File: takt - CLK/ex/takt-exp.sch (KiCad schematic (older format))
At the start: 55 parts, among them J1 PJ301M-12, J2 PJ301M-12, J3 PJ301M-12, J4 PJ301M-12, J5 PJ301M-12, J6 PJ301M-12, J7 PJ301M-12, J8 PJ301M-12, J9 PJ301M-12, Q1 2N3904, Q2 2N3904, Q3 2N3904, SW1 SW_SP3T, SW2 SW_SP3T, SW3 SW_SP3T, U1 TL074, U2 TL074, U3 TL074, U4 ATmega328P-PU

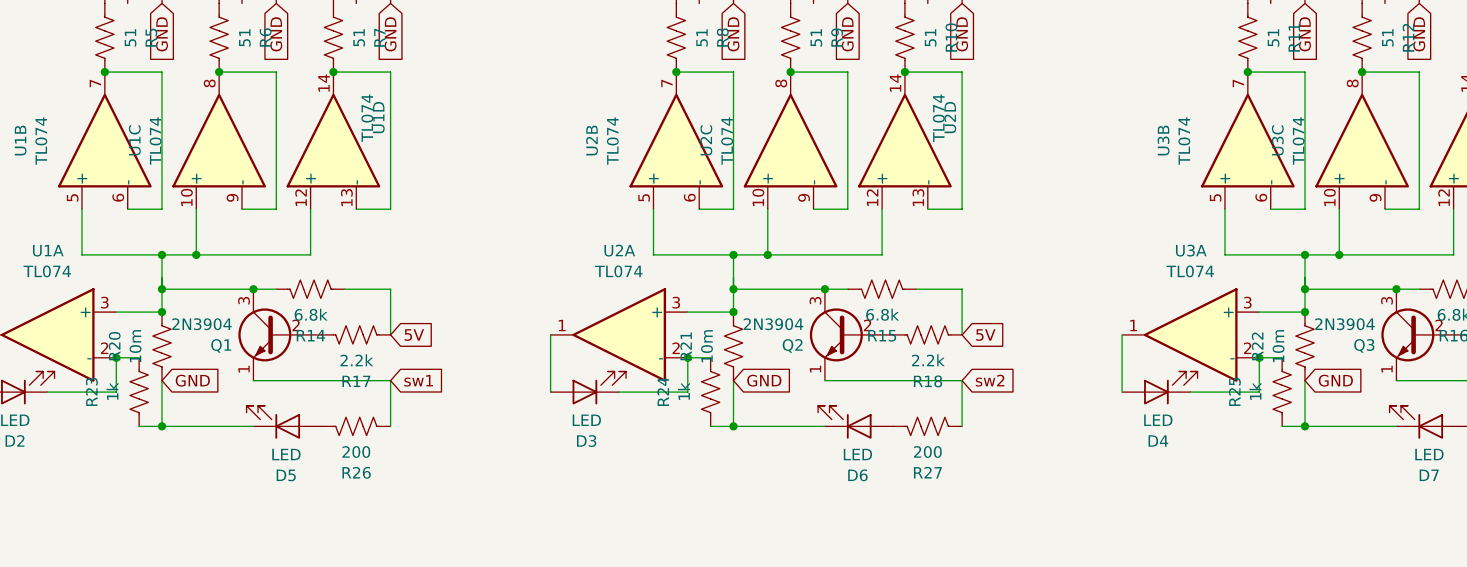
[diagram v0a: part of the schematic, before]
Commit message: update
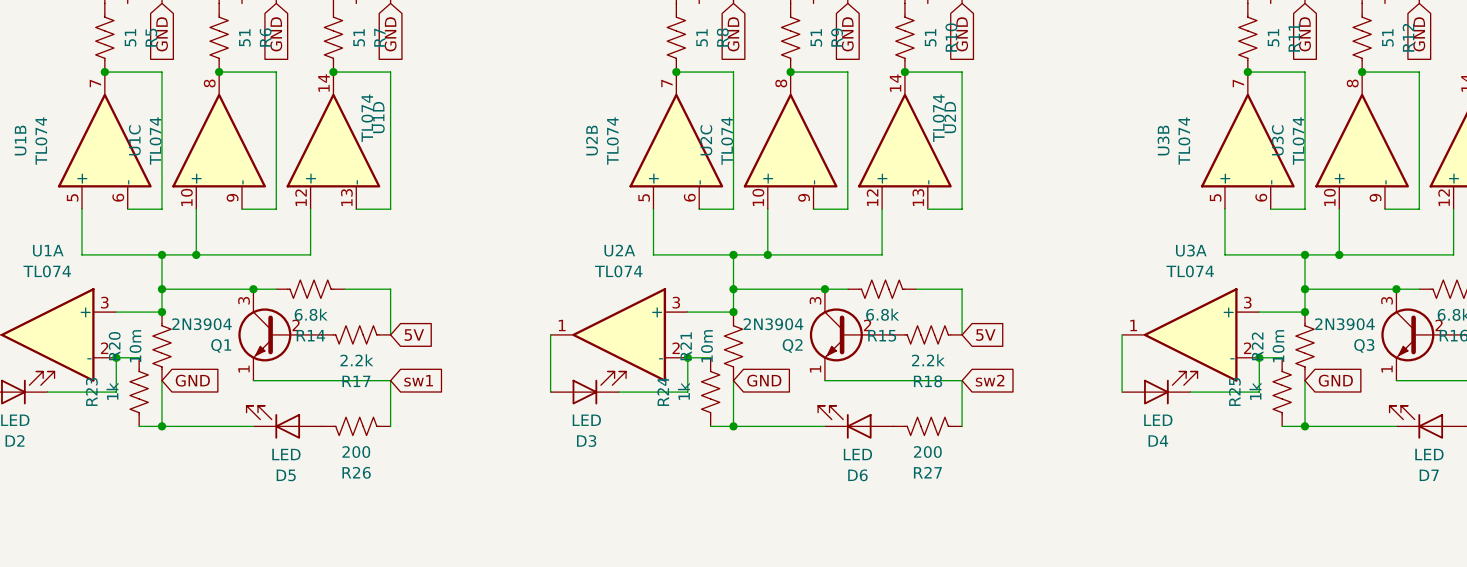
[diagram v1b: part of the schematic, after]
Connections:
- wire segments 102 -> 99
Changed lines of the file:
@@
 Tr9
-Wire Wire Line
-	1550 3400 1550 3450
-Wire Wire Line
-	4050 3400 4050 3450
-Wire Wire Line
-	6550 3400 6550 3450
 Wire Wire Line
 	1550 3300 1550 3450
